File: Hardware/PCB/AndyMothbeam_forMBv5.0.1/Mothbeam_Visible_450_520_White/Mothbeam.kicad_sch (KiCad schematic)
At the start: 26 parts, among them CN1 X6511FRS-04-C85D30, SW2 SW_DIP_x04, U1 BCR421U, U2 BCR421U, U3 BCR421U, U4 M3535N1UVS8U12- 405NM, U5 M3535N1UVS8U06-385NM

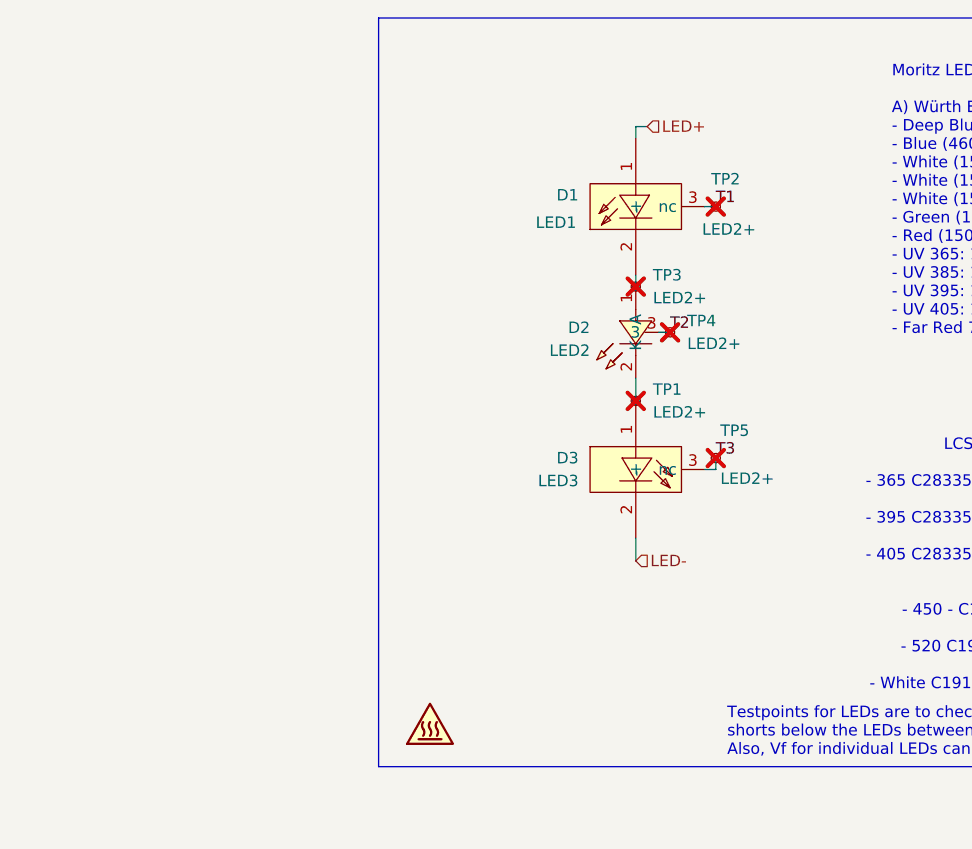
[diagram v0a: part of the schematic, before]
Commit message: before changing footprints on Visible board
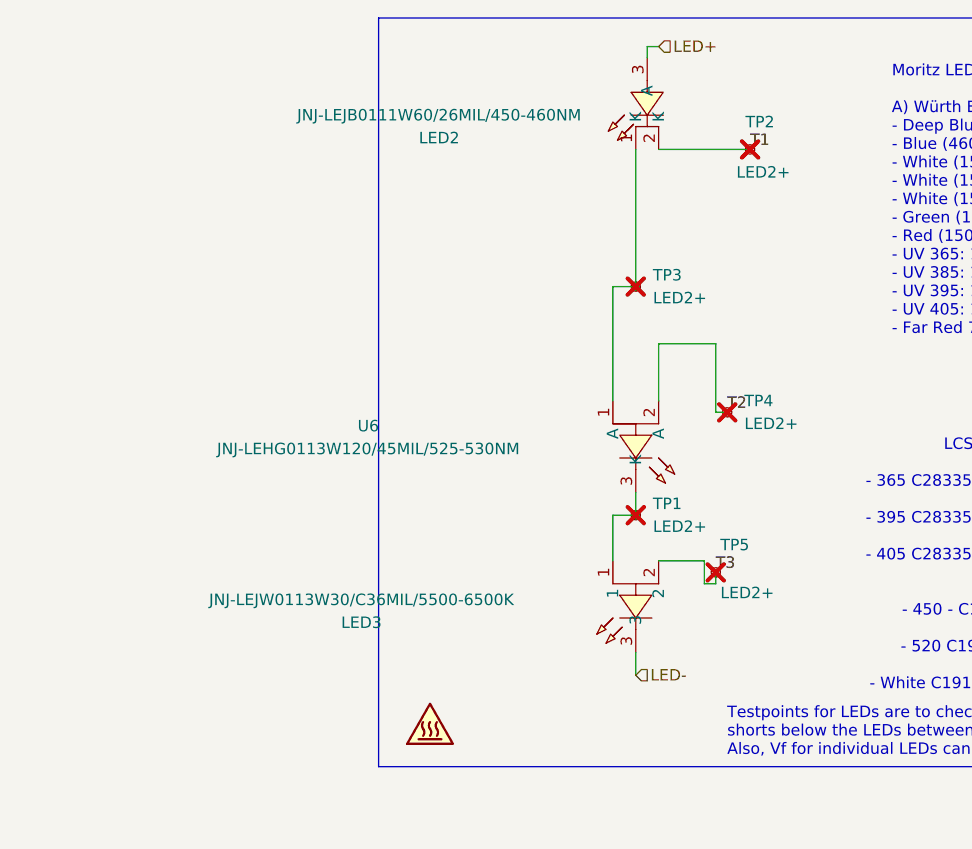
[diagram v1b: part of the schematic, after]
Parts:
- removed D1: LED1, easyeda2kicad:LED-SMD_3P-L3.5-W3.5-R-RD-C, symbol easyeda2kicad:M3535N1UVS8U12-365NM
- removed D2: LED2, easyeda2kicad:LED-SMD_3P-L3.5-W3.5-R-RD-C, symbol easyeda2kicad:M3535N1UVS8U12-395NM
- removed D3: LED3, easyeda2kicad:LED-SMD_3P-L3.5-W3.5-R-RD-C, symbol easyeda2kicad:M3535N1UVS8U12-405NM
- added LED2: JNJ-LEJB0111W60/26MIL/450-460NM, easyeda2kicad:LED-SMD_3P-L3.5-W3.5_JNJ-LEJB0111W60, symbol easyeda2kicad:JNJ-LEJB0111W60_26MIL_450-460NM
- added LED3: JNJ-LEJW0113W30/C36MIL/5500-6500K, easyeda2kicad:LED-SMD_3P-L3.5-W3.5-R-RD-B, symbol easyeda2kicad:JNJ-LEJW0113W30_C36MIL_5500-6500K
- added U6: JNJ-LEHG0113W120/45MIL/525-530NM, easyeda2kicad:LED-SMD_3P-L3.5-W3.5-R-RD_C9900043159, symbol easyeda2kicad:JNJ-LEHG0113W120_45MIL_525-530NM
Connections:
- net LED+: now also LED2.3 (A)
- net LED-: now also LED3.3
- net T1: now also LED2.2 (K)
- net T2: now also U6.2 (A)
- net T3: now also LED3.2
- net at TP3.1: now also LED2.1 (K), U6.1 (A)
- net at TP1.1: now also LED3.1, U6.3 (K)
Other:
- moved on the sheet: TP1, TP2, TP4, TP5
